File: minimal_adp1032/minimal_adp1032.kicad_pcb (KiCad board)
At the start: 4 copper layers, 35.6 x 39.6 mm, 60 parts, among them J1 FW-07-03-G-D-085-155, J2 FW-07-03-G-D-085-155, J3 FW-02-03-G-D-085-155, J4 FW-02-03-G-D-085-155, J5 FW-02-03-G-D-085-155, J6 FW-02-03-G-D-085-155, T1 ZA9644-AED, U1 ADP1032ACPZ-5-R7

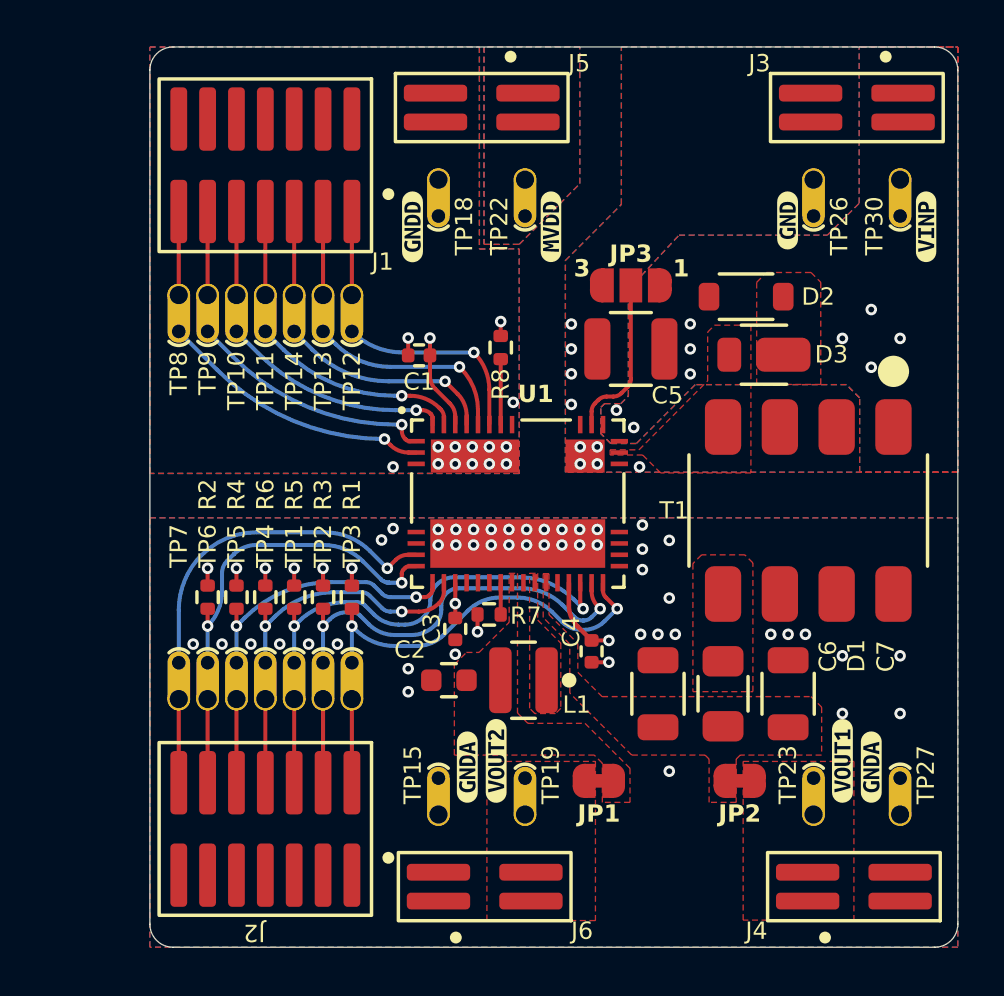
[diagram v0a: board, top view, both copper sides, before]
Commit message: Minor updates
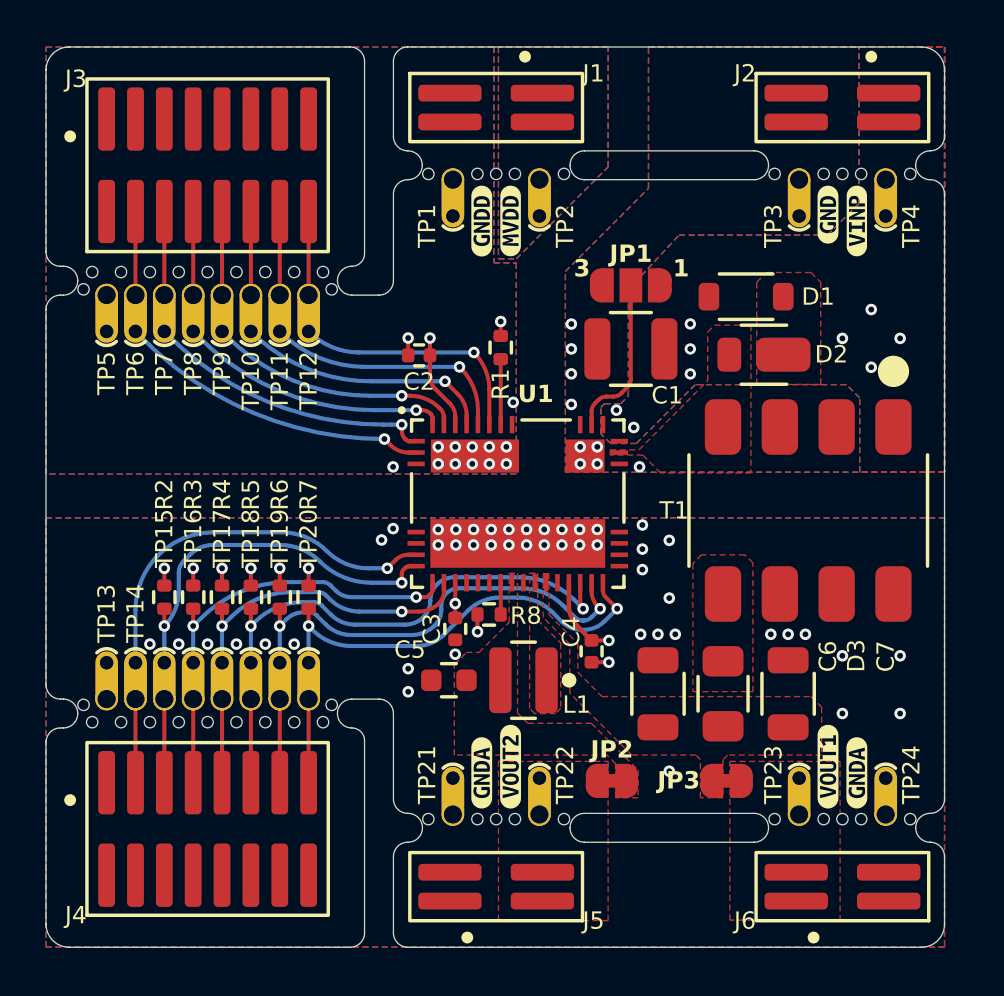
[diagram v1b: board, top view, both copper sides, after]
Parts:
- added REF**: mouse-bite-50mil-305mil, mouse_bite_footprints:mouse-bite-50mil-305mil, F.Cu at (151.8, 117.4)
- added REF**: mouse-bite-50mil-305mil, mouse_bite_footprints:mouse-bite-50mil-305mil, F.Cu at (151.8, 88.3)
- added REF**: mouse-bite-50mil-500mil, mouse_bite_footprints:mouse-bite-50mil-500mil, F.Cu at (139.1, 93.5)
- added REF**: mouse-bite-50mil-500mil, mouse_bite_footprints:mouse-bite-50mil-500mil, F.Cu at (139.1, 112.3)
- added REF**: mouse-bite-50mil-305mil, mouse_bite_footprints:mouse-bite-50mil-305mil, F.Cu at (167.0, 117.4)
- added REF**: mouse-bite-50mil-305mil, mouse_bite_footprints:mouse-bite-50mil-305mil, F.Cu at (167.0, 88.3)
- added TP13: TestPoint, test_point_footprints:TestPoint_THTPad_Castelated, F.Cu at (134.6, 111.8)
- added TP5: TestPoint, test_point_footprints:TestPoint_THTPad_Castelated, F.Cu at (134.6, 94.0)
- J3: renamed from J1; footprint connector_footprints:FW-07-03-G-D-085-155 -> connector_footprints:FW-08-03-G-D-085-155
- J4: renamed from J2; footprint connector_footprints:FW-07-03-G-D-085-155 -> connector_footprints:FW-08-03-G-D-085-155
- moved kibuzzard-4 3.06 mm to (167.6, 90.7)
- moved kibuzzard-2 3.06 mm to (151.1, 90.7)
- moved J3 2.54 mm to (139.1, 88.3), turned to 0 degrees
- moved J4 2.54 mm to (139.1, 117.5), turned to 0 degrees
- moved R2 1.91 mm to (137.2, 107.3)
- moved R3 1.91 mm to (138.4, 107.3)
- moved R4 1.91 mm to (139.7, 107.3)
- moved R5 1.91 mm to (141.0, 107.3)
- moved R6 1.91 mm to (142.2, 107.3)
- moved R7 1.91 mm to (143.5, 107.3)
- moved TP10 1.91 mm to (141.0, 94.0)
- moved TP11 1.91 mm to (142.2, 94.0)
- moved TP12 1.91 mm to (143.5, 94.0)
- moved TP14 1.91 mm to (135.9, 111.8)
- moved TP15 1.91 mm to (137.2, 111.8)
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- renumbered C5 to C1, C1 to C2, C2 to C5, D2 to D1, D3 to D2, D1 to D3, J5 to J1, J3 to J2, J6 to J5, J4 to J6, JP3 to JP1, JP1 to JP2, JP2 to JP3, R8 to R1, R4 to R3, R6 to R4, R3 to R6, R1 to R7, R7 to R8, TP18 to TP1, TP14 to TP10, TP13 to TP11, TP7 to TP14, TP6 to TP15, TP5 to TP16, TP4 to TP17, TP1 to TP18, TP2 to TP19, TP22 to TP2, TP3 to TP20, TP15 to TP21, TP19 to TP22, TP27 to TP24, TP26 to TP3, TP30 to TP4, TP8 to TP6, TP9 to TP7, TP10 to TP8, TP11 to TP9, kibuzzard-678A0FCE to kibuzzard-1, kibuzzard-679E3671 to kibuzzard-2, kibuzzard-678A0F1C to kibuzzard-3, kibuzzard-678A0FC5 to kibuzzard-4, kibuzzard-679E35DB to kibuzzard-5, kibuzzard-678A1049 to kibuzzard-6, kibuzzard-678A0E06 to kibuzzard-7, kibuzzard-678A1052 to kibuzzard-8
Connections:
- J3 pad 1: /MGPI1 -> GNDD
- J3 pad 10: GNDD -> /MCK
- J3 pad 11: /MI -> GNDD
- J3 pad 12: GNDD -> /MGPO3
- J3 pad 13: /~{MSS} -> GNDD
- J3 pad 14: GNDD -> /MGPI2
- J3 pad 3: /MGPI2 -> GNDD
- J3 pad 4: GNDD -> /~{MSS}
- J3 pad 5: /MGPO3 -> GNDD
- J3 pad 6: GNDD -> /MI
- J3 pad 7: /MCK -> GNDD
- J3 pad 8: GNDD -> /MO
- J3 pad 9: /MO -> GNDD
- J4 pad 10: /SI -> GNDA
- J4 pad 11: GNDA -> /SGPI3
- J4 pad 12: /SO -> GNDA
- J4 pad 13: GNDA -> /SPGO2
- J4 pad 14: /~{SSS} -> GNDA
- J4 pad 2: /SPGO1 -> GNDA
- J4 pad 3: GNDA -> /~{SSS}
- J4 pad 4: /SPGO2 -> GNDA
- J4 pad 5: GNDA -> /SO
- J4 pad 6: /SGPI3 -> GNDA
- J4 pad 7: GNDA -> /SI
- J4 pad 8: /SCK -> GNDA
- J4 pad 9: GNDA -> /SCK
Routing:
- net /MGPI1: track 12.6 -> 14.5 mm
- net /SPGO2: track 21.8 -> 23.7 mm
- net /SPGO1: track 20.8 -> 22.7 mm
- net /SGPI3: track 22.1 -> 24.0 mm
- net /SI: track 15.9 -> 17.8 mm
- net /SCK: track 15.5 -> 17.3 mm
- net /MGPI2: track 12.9 -> 14.7 mm
- net /MCK: track 13.1 -> 14.9 mm
- net /MO: track 13.8 -> 15.6 mm
- net /~{SSS}: track 19.1 -> 20.9 mm
- net /MGPO3: track 13.2 -> 15.0 mm
- net /SO: track 18.8 -> 20.6 mm
- net /MI: track 14.6 -> 16.4 mm
- net /~{MSS}: track 15.8 -> 17.5 mm
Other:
- board size 35.6 x 39.6 mm -> 39.5 x 39.6 mm
